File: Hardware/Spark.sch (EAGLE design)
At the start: 8 parts

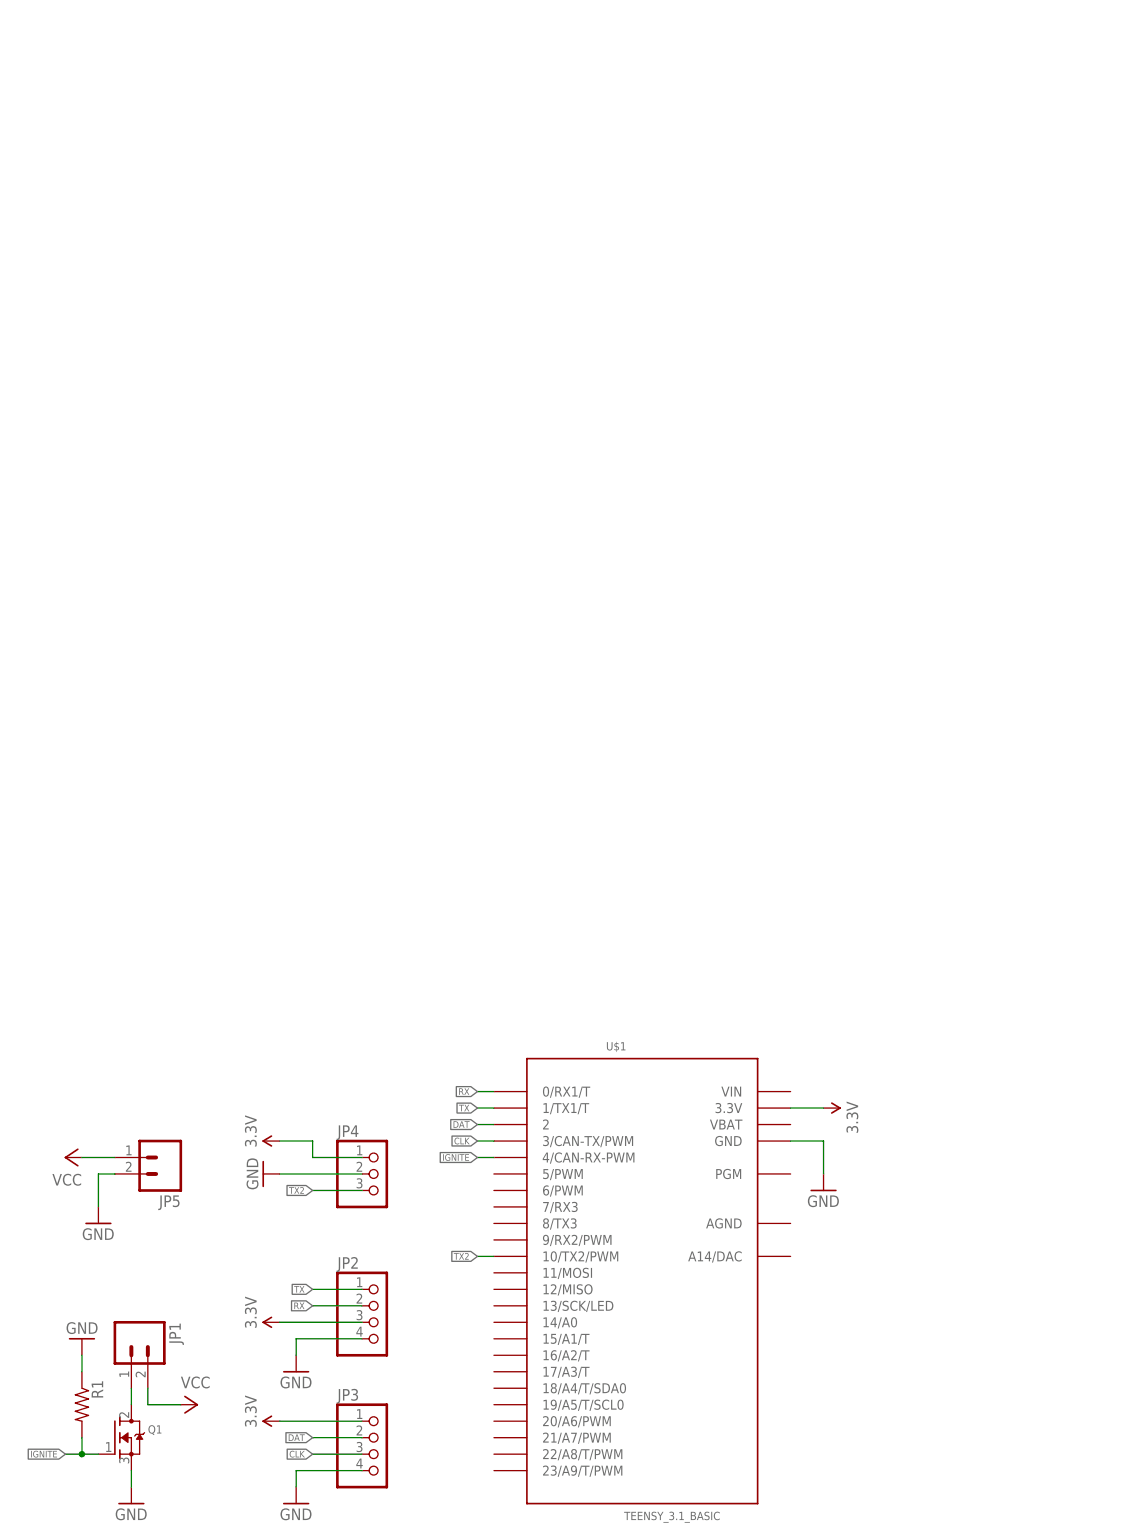
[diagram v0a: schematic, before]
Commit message: begin v2
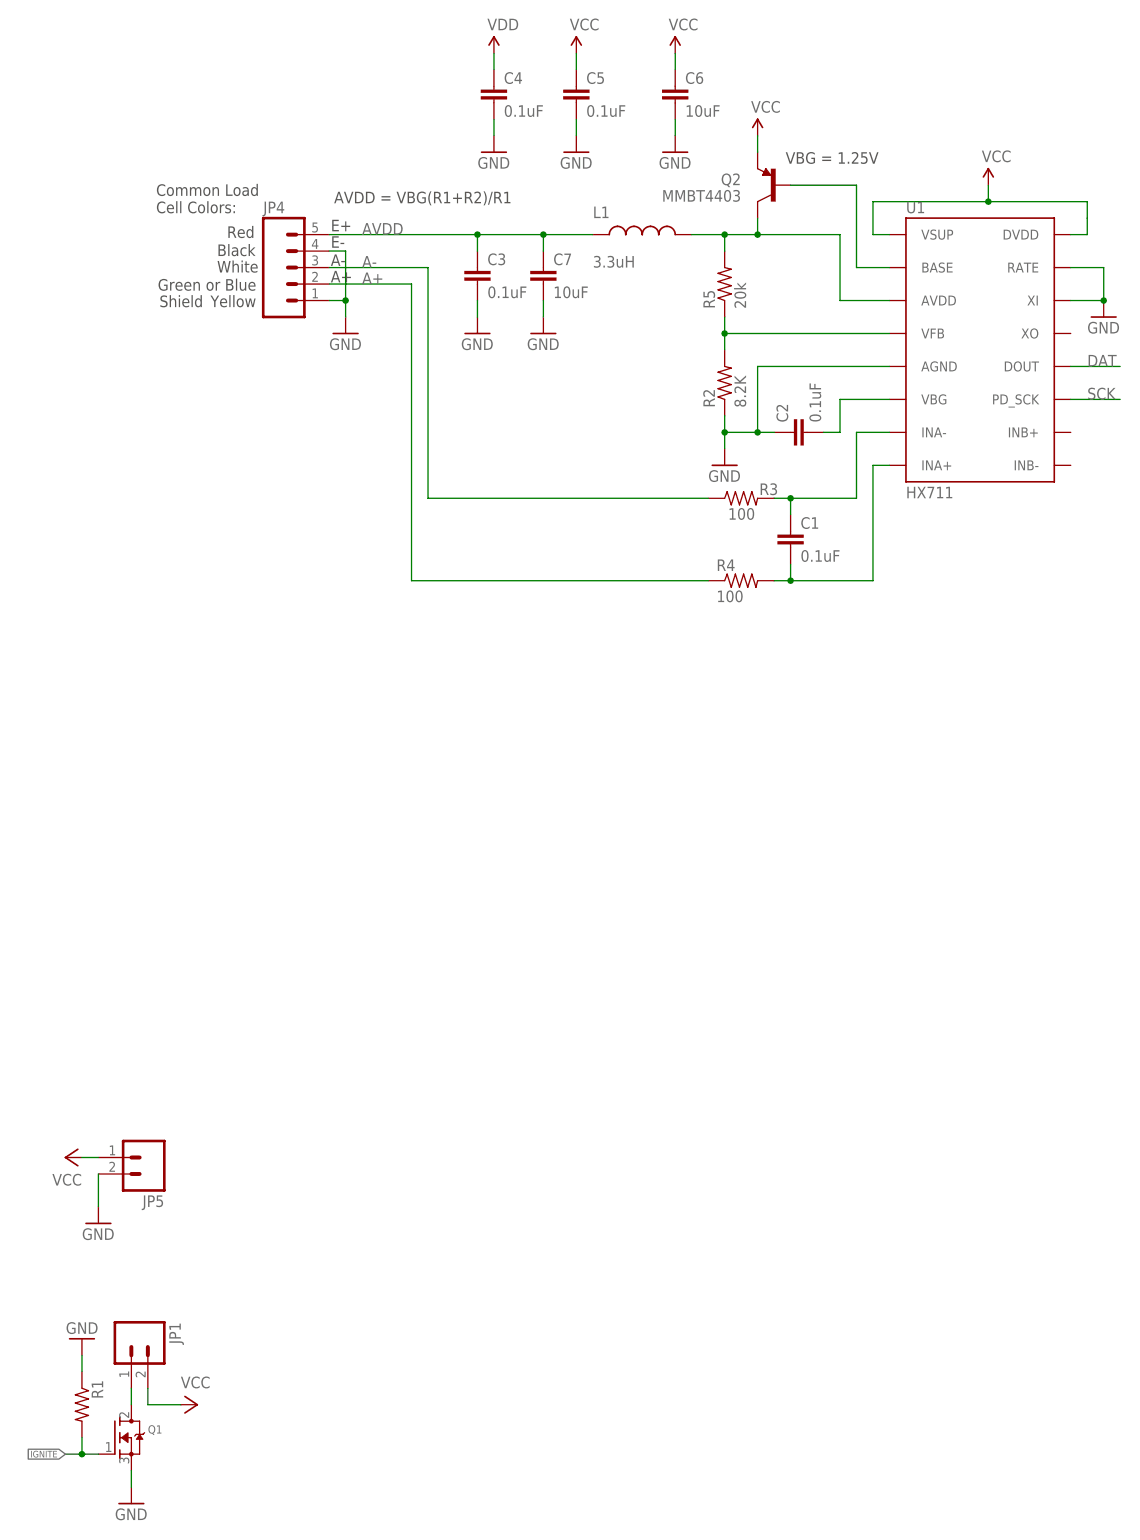
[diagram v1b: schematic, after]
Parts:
- removed JP2, JP3: (no value), pinhead:PINHD-1X4
- removed U$1: TEENSY_3.1_BASIC, Teensy_3_Series_Board_v1.0:TEENSY_3.1_BASIC
- added C1, C2, C3, C4, C5: 0.1uF, SparkFun-Capacitors:0.1UF-25V-5%(0603)
- added C6, C7: 10uF, SparkFun-Capacitors:10UF50V20%(1210)
- added L1: 3.3uH, SparkFun-Passives:INDUCTOR0805
- added Q2: MMBT4403, SparkFun-DiscreteSemi:TRANSISTOR_PNPMMBT4403
- added R2: 8.2K, SparkFun-Resistors:8.2KOHM-1/10W-5%(0603)
- added R3, R4: 100, SparkFun-Resistors:100OHM-1/10W-1%(0603)
- added R5: 20k, SparkFun-Resistors:20KOHM1/10W1%(0603)
- added U1: HX711, Testing:HX711HX711
- JP4: device pinhead:PINHD-1X3 -> SparkFun-Connectors:M05PTH
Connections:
- removed net 3.3V: JP2.3, JP3.1, JP4.1, U$1.3.3V
- removed net CLK: JP3.3, U$1.3/CAN-TX/PWM
- removed net RX: JP2.2, U$1.0/RX1/T
- removed net TX: JP2.1, U$1.1/TX1/T
- removed net TX2: JP4.3, U$1.10/TX2/PWM
- new net A+: JP4.2, R4.1
- new net A-: JP4.3, R3.1
- new net AVDD: C3.1, C7.1, JP4.5, L1.1
- new net N$10: U1.DVDD
- new net N$3: C1.1, R3.2, U1.INA-
- new net N$4: Q2.B, U1.BASE
- new net N$5: L1.2, Q2.C, R5.2, U1.AVDD
- new net N$6: R2.2, R5.1, U1.VFB
- new net N$7: C2.2, U1.VBG
- new net N$8: C1.2, R4.2, U1.INA+
- new net SCK: U1.PD_SCK
- new net VDD: C4.1
- net DAT: now also U1.DOUT; no longer JP3.2, U$1.2
- net GND: now also C2.1, C3.2, C4.2, C5.2, C6.2, C7.2, JP4.1, JP4.4, R2.1, U1.AGND, U1.RATE, U1.XI; no longer JP2.4, JP3.4, JP4.2, U$1.GND
- net IGNITE: no longer U$1.4/CAN-RX-PWM
- net VCC: now also C5.1, C6.1, Q2.E, U1.VSUP
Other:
- note added: "A+"
- note added: "A-"
- note added: "AVDD = VBG(R1+R2)/R1"
- note added: "Black"
- note added: "Common Load Cell Colors:"
- note added: "E+"
- note added: "E-"
- note added: "Green or Blue"
- note added: "Red"
- note added: "Shield"
- note added: "VBG = 1.25V"
- note added: "White"
- note added: "Yellow"
- moved on the sheet: JP5
